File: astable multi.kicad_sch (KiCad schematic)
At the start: 9 parts, among them Q1 NPN, Q2 Q_NPN_EBC

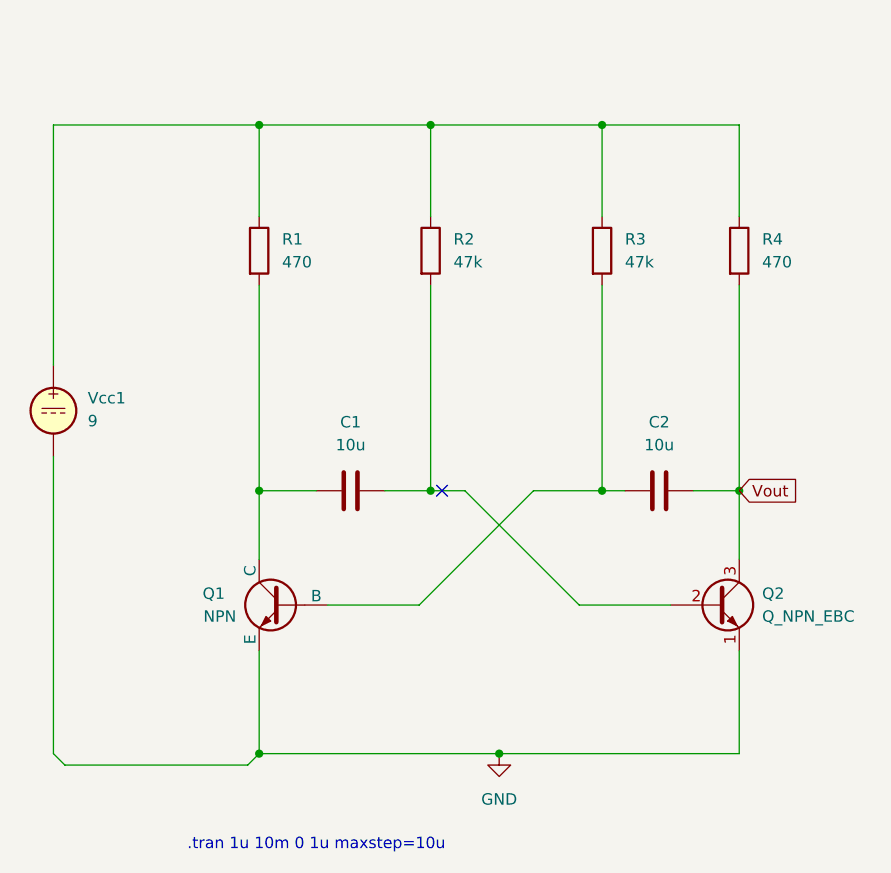
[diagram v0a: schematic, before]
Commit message: third commit
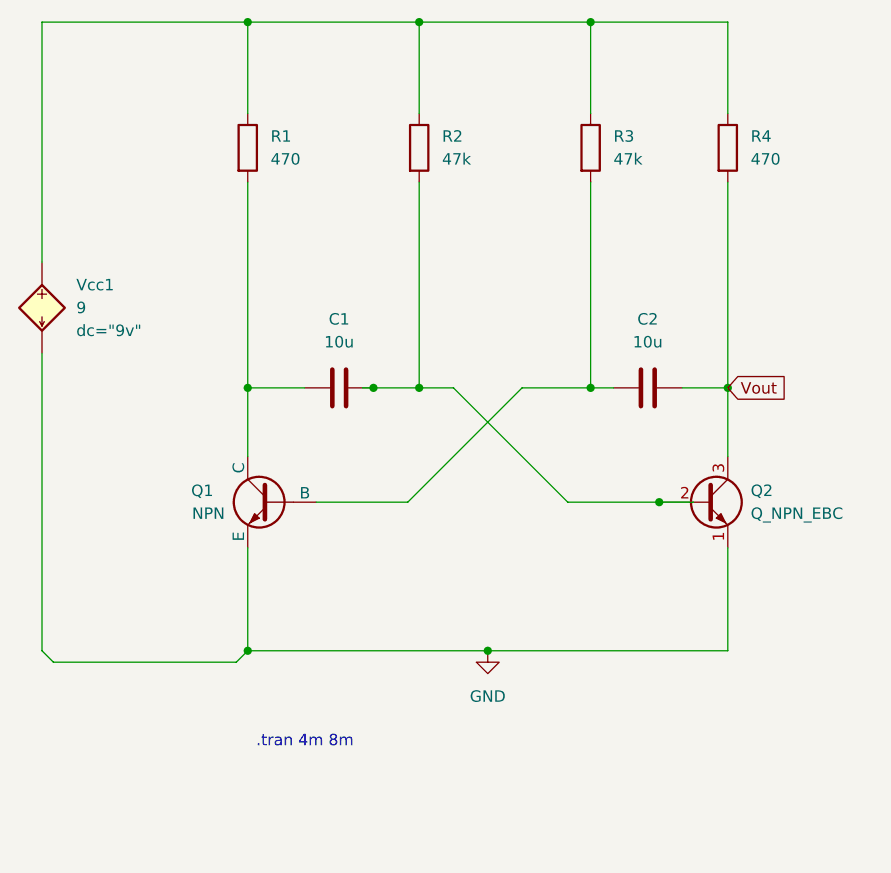
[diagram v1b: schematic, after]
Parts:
- removed Vcc1: 9, symbol Simulation_SPICE:VDC
- added Vcc1: 9, symbol Simulation_SPICE:BSOURCE
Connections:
- net GND: now also Vcc1.2 (N-)
- net at R1.1, R2.1, R3.1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: now also Vcc1.1 (N+)
- no-connect marks 1 -> 0
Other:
- note added: ".tran 4m 8m"
- note removed: ".tran 1u 10m 0 1u maxstep=10u"
- moved on the sheet: C1, C2, Q1, Q2, R1, R2, R3, R4
